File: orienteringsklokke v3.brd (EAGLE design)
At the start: 40.8 x 50 mm, 16 parts

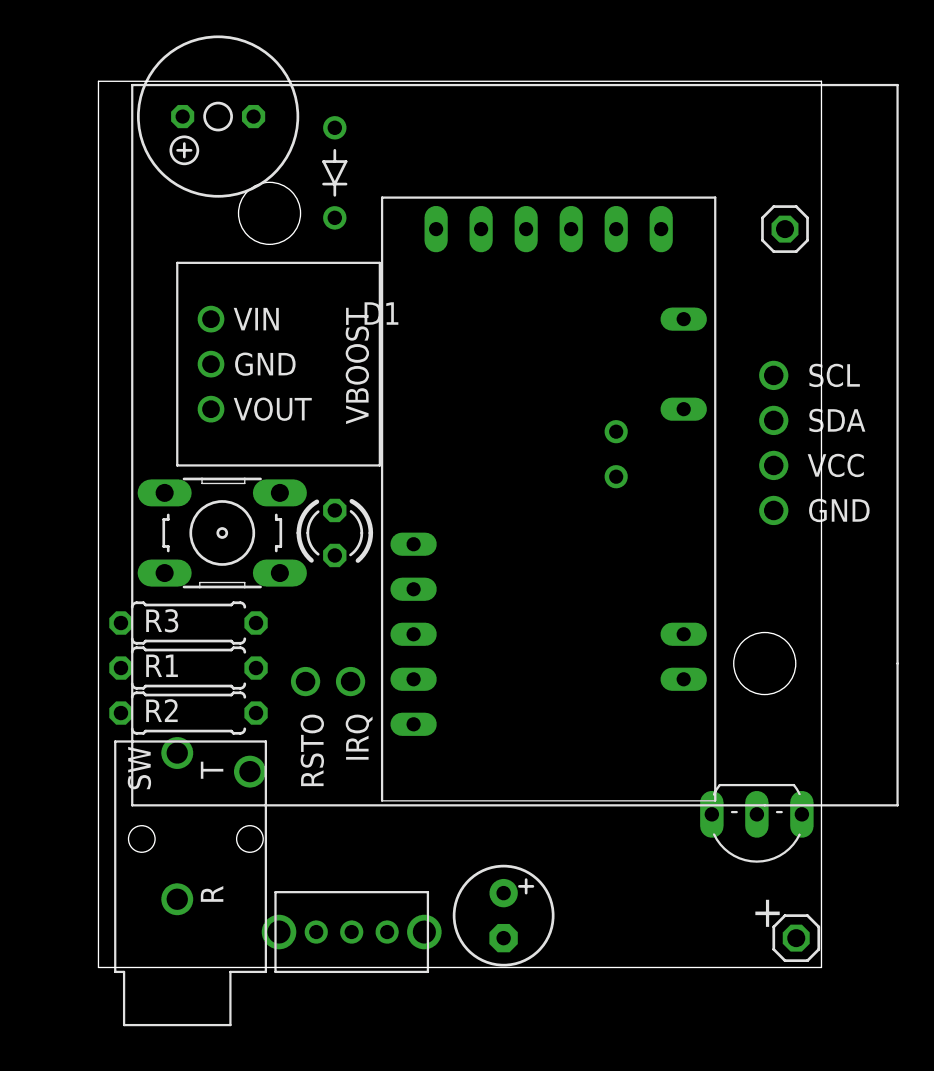
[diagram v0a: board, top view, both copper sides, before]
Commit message: Lots of work on version 3
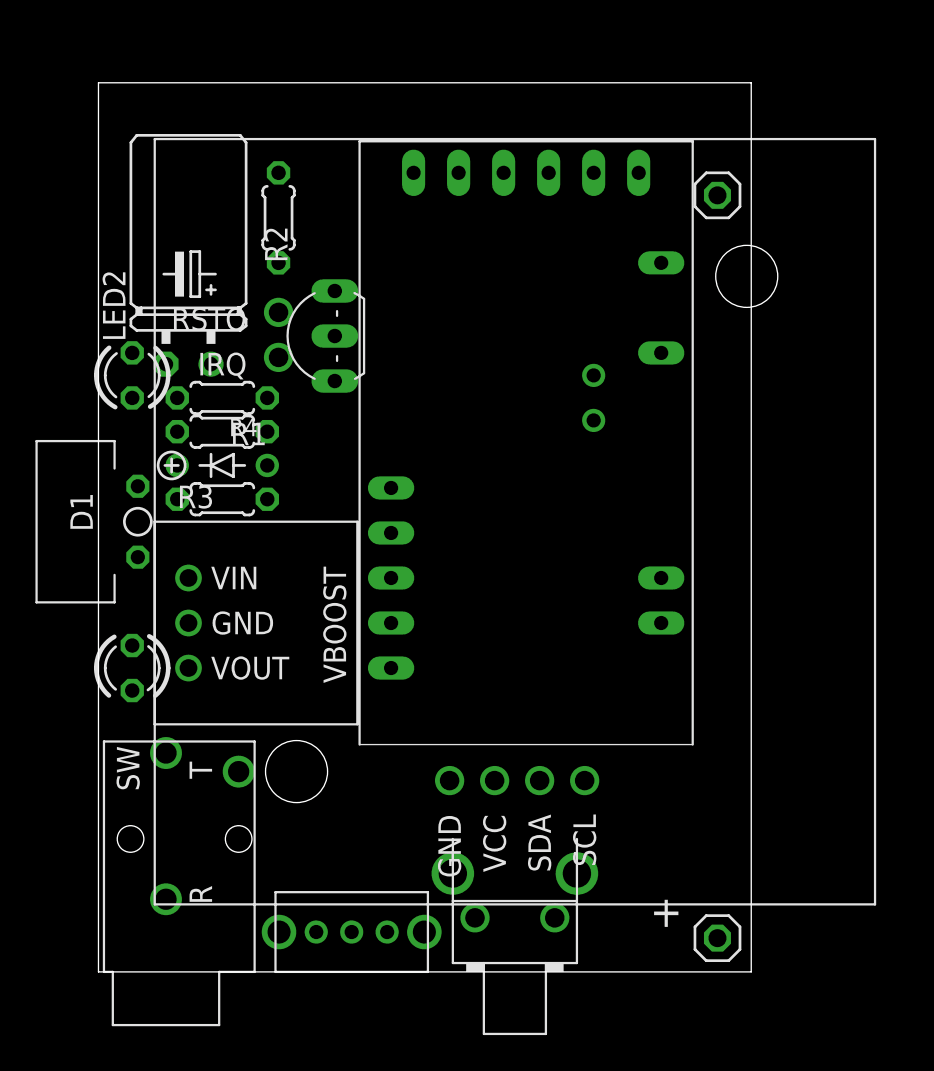
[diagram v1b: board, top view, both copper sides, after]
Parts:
- removed S1: (no value), switch-omron:B3F-10XX
- added LED2: (no value), led:LED3MM
- added R4: 220, resistor:0204/5
- added U$5: PUSHBUTTON_2P, joakim:PUSHBUTTON_HORIZ_J
- C1: device resistor:E2,5-6 -> joakim:CAP-HORIZ-6.5X11X2.5
- R1, R2, R3: device resistor:0207/7 -> resistor:0204/5
- U$1: value BUZZER_J -> BUZZER_JL; device joakim:BUZZER_J -> joakim:BUZZER_HORIZ_J_LEFT
- U$2: value NFC_MODULE_V3_I2C -> NFC_MODULE_V3_I2CC; device joakim:NFC_MODULE_V3_I2C -> joakim:NFC_MODULE_V3_I2C_CENTERED
- moved T1 37.8 mm to (12.1, 35.9), turned to 90 degrees
- moved C1 35.8 mm to (5.08, 34.3), turned to 90 degrees
- moved R2 28.4 mm to (10.2, 42.5), turned to 270 degrees
- moved U$1 25.0 mm to (-3.49, 25.4), turned to 90 degrees
- moved D1 17.7 mm to (6.99, 28.6), turned to 0 degrees
- moved U$3 14.7 mm to (5.08, 19.7)
- moved U$2 14.6 mm to (23.5, 25.4), turned to 90 degrees
- moved LED1 13.7 mm to (1.91, 17.1)
- moved R1 13.5 mm to (6.99, 30.5), turned to 180 degrees
- moved R3 7.24 mm to (6.99, 26.7)
- moved BATTERY_VCC 4.45 mm to (34.9, 1.91)
- moved BATTERY_GND 4.26 mm to (34.9, 43.8)
- moved U$4 3.42 mm to (24.1, 29.8)
- moved CHARGE 0.64 mm to (3.81, 0.00)
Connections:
- net LED renamed LED1
- new net LED2: R4.1
- new net N$8: LED2.A, R4.2
- net GND: now also LED2.K, U$5.2; no longer S1.4
- net SWITCH: now also U$5.1; no longer S1.1
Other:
- board size 40.8 x 50 mm -> 36.8 x 50.2 mm
- board text added: "Husk overgang mellom side og batterikontakt"

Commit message: Hopefully final layout, tracing left
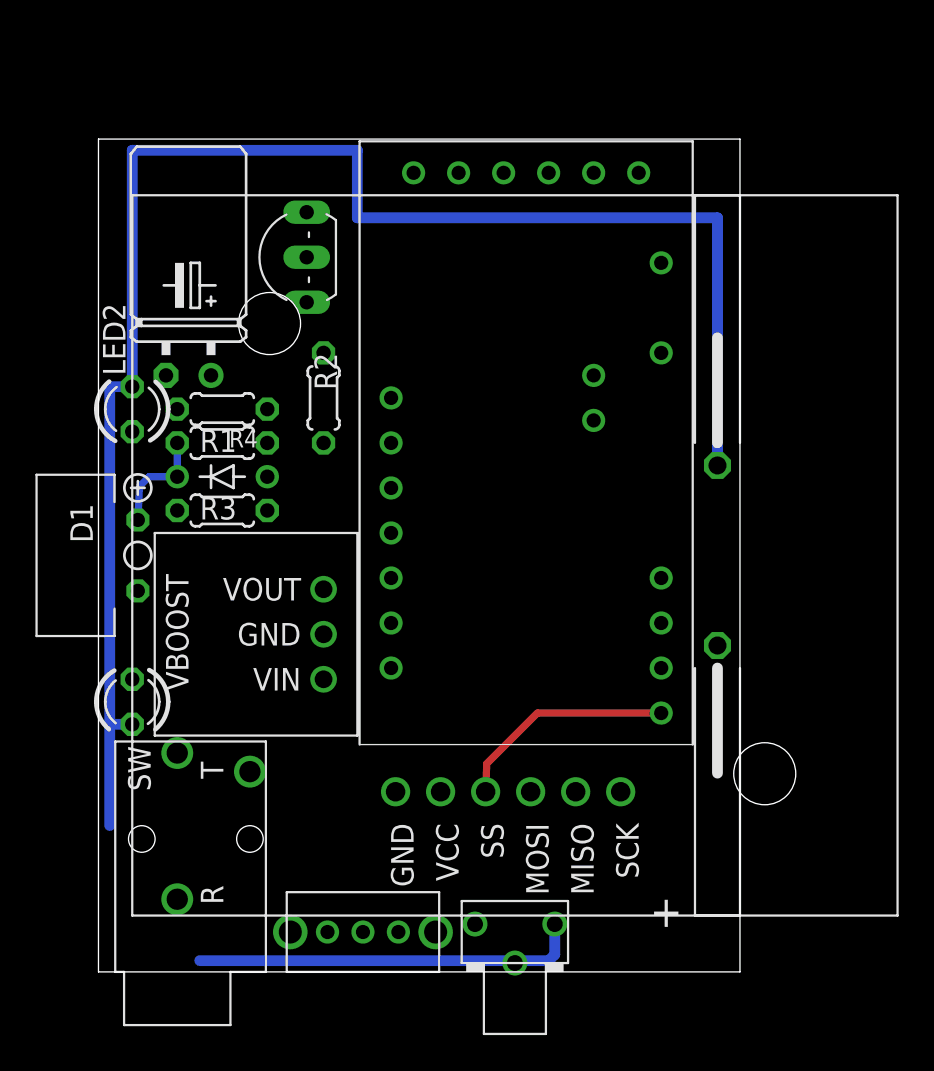
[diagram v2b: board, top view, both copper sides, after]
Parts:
- BATTERY_GND, BATTERY_VCC: value (none) -> DUPONT-PIN-90DEG; device joakim:MA01-1J -> joakim:DUPONT-PIN-90DEG
- R1: value 100 -> 68
- U$2: value NFC_MODULE_V3_I2CC -> NFC_MODULE_V3_SPI; device joakim:NFC_MODULE_V3_I2C_CENTERED -> joakim:NFC_MODULE_V3_SPI_CENTERED
- U$5: value PUSHBUTTON_2P -> PUSHBUTTON_2P6MM; device joakim:PUSHBUTTON_HORIZ_J -> joakim:PUSHBUTTON_HORIZ_6MM_J
- moved BATTERY_VCC 16.5 mm to (34.9, 18.4)
- moved BATTERY_GND 15.2 mm to (34.9, 28.6), turned to 180 degrees
- moved R2 10.5 mm to (12.7, 32.4), turned to 90 degrees
- moved U$3 7.65 mm to (12.7, 19.1), turned to 90 degrees
- moved T1 4.72 mm to (10.5, 40.3)
- moved LED2 1.91 mm to (1.91, 31.8)
- moved LED1 1.90 mm to (1.91, 15.2)
- moved U$1 1.90 mm to (-3.49, 23.5)
- moved U$2 1.90 mm to (23.5, 23.5), turned to 180 degrees
- moved R1 0.64 mm to (6.99, 29.8)
- moved R3 0.64 mm to (6.99, 26.0)
- moved CHARGE 0.64 mm to (4.45, 0.00)
- moved U$6 0.63 mm to (14.9, 0.00)
- moved C1 0.63 mm to (5.08, 33.7)
- moved D1 0.63 mm to (6.99, 27.9)
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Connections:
- removed net IRQ: U$2.IRQ, U$4.D7
- removed net RSTO: U$2.RSTO, U$4.D8
- new net MISO: U$2.MISO, U$4.D12
- new net MOSI: U$2.MOSI, U$4.D11
- new net SCK: U$2.SCK, U$4.D13
- new net SS: U$2.SS, U$4.D10
- net BUZZER: now also U$4.D3; no longer U$4.D6
- net LED2: now also U$4.D2
- net SCL: no longer U$2.SCL
- net SDA: no longer U$2.SDA
- net SWITCH: now also U$4.D8; no longer U$4.D5
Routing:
- net GND: track 0.00 -> 113.3 mm
- net SS: track 0.00 -> 12.6 mm
- net N$4: track 0.00 -> 6.16 mm
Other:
- board size 36.8 x 50.2 mm -> 36.2 x 47 mm
- board text removed: "Husk overgang mellom side og batterikontakt"
